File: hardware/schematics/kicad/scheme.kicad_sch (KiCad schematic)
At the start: 15 parts, among them J1 RJ45, J2 RJ45, J3 RJ45

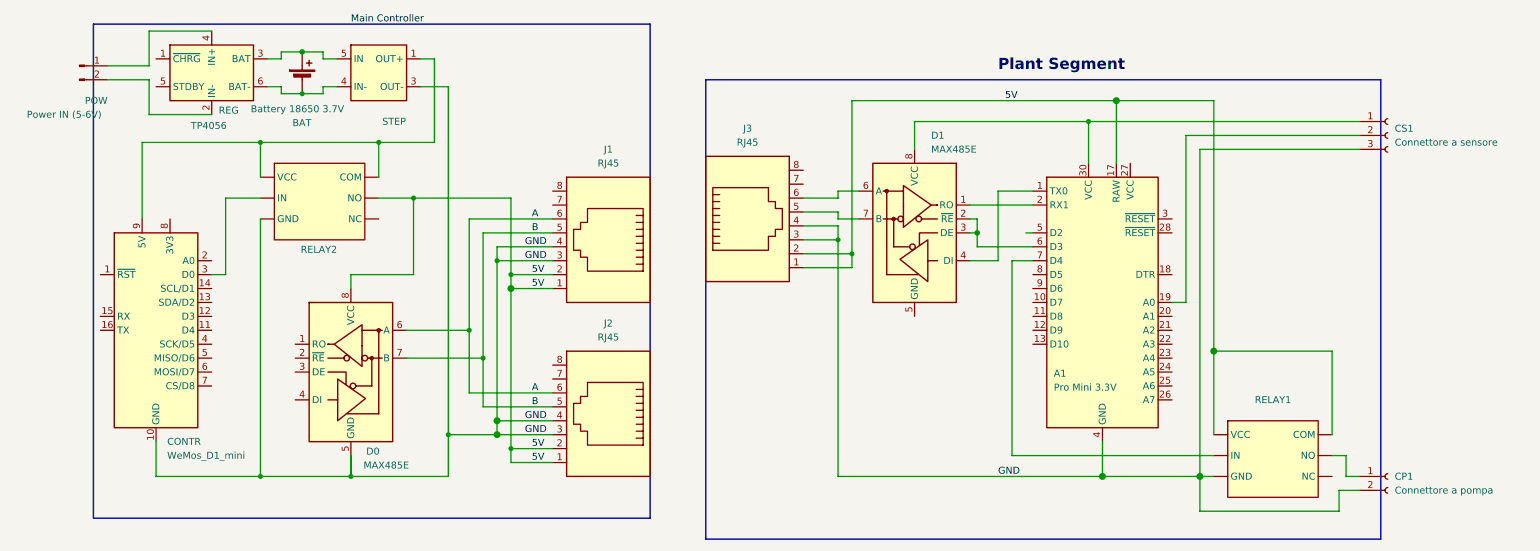
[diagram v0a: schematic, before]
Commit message: saved schematics & formatted
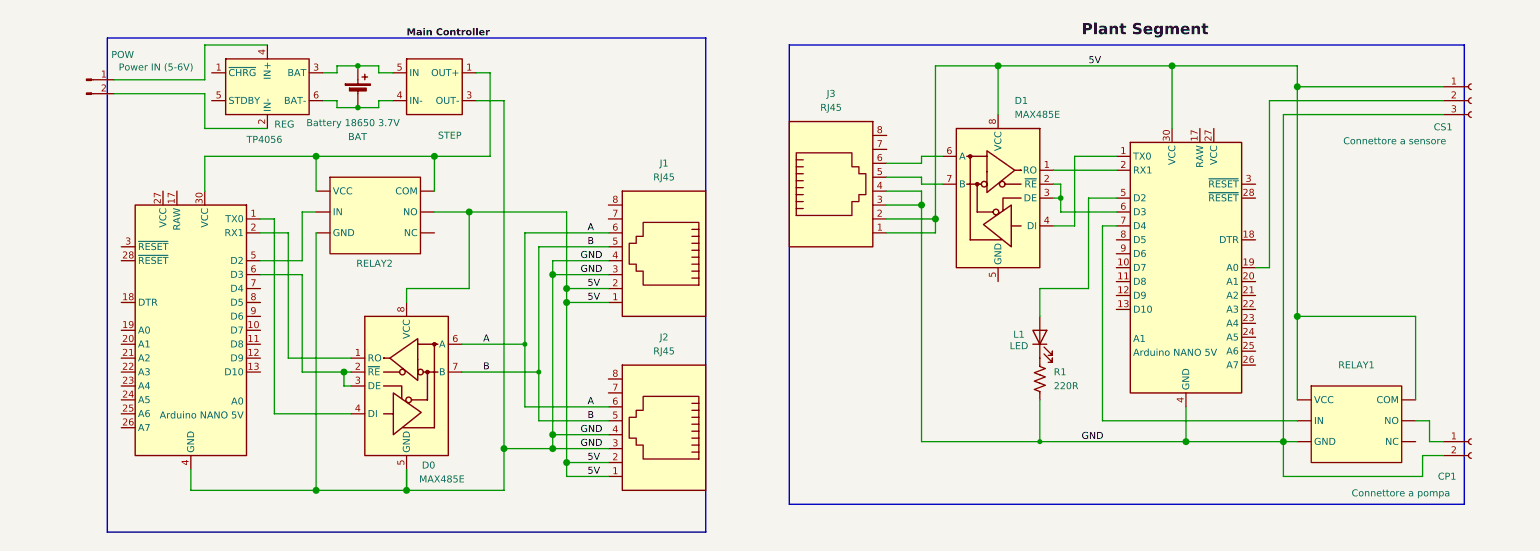
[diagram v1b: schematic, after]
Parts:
- removed CONTR: WeMos_D1_mini, Module:WEMOS_D1_mini_light, symbol MCU_Module:WeMos_D1_mini
- added A0: Arduino NANO 5V, symbol MCU_Module:Arduino_Nano_Every
- added L1: LED, symbol Device:LED
- added R1: 220R, symbol Device:R_US
- A1: value Pro Mini 3.3V -> Arduino NANO 5V
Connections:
- net 5V: now also A1.30 (VCC), CS1.1 (Pin_1), D1.8 (VCC); no longer A1.17 (RAW)
- net GND: now also A0.29 (GND), A0.4 (GND), R1.2
- net at RELAY2. (VCC), STEP.1 (OUT+): now also A0.30 (VCC)
- net at D0.1 (RO): now also A0.2 (RX1)
- net at D0.2 (~{RE}): now also D0.3 (DE), A0.6 (D3)
- net at D0.4 (DI): now also A0.1 (TX0)
- net at A1.5 (D2): now also L1.2 (A)
- new net: L1.1 (K), R1.1
- new net: A0.5 (D2), RELAY2. (VCC)
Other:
- moved on the sheet: A1, BAT, CP1, CS1, D0, D1, J1, J2, J3, POW, REG, RELAY1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
